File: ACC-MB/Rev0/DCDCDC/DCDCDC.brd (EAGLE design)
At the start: 99 x 78 mm, 20 parts, among them X5 5566-8

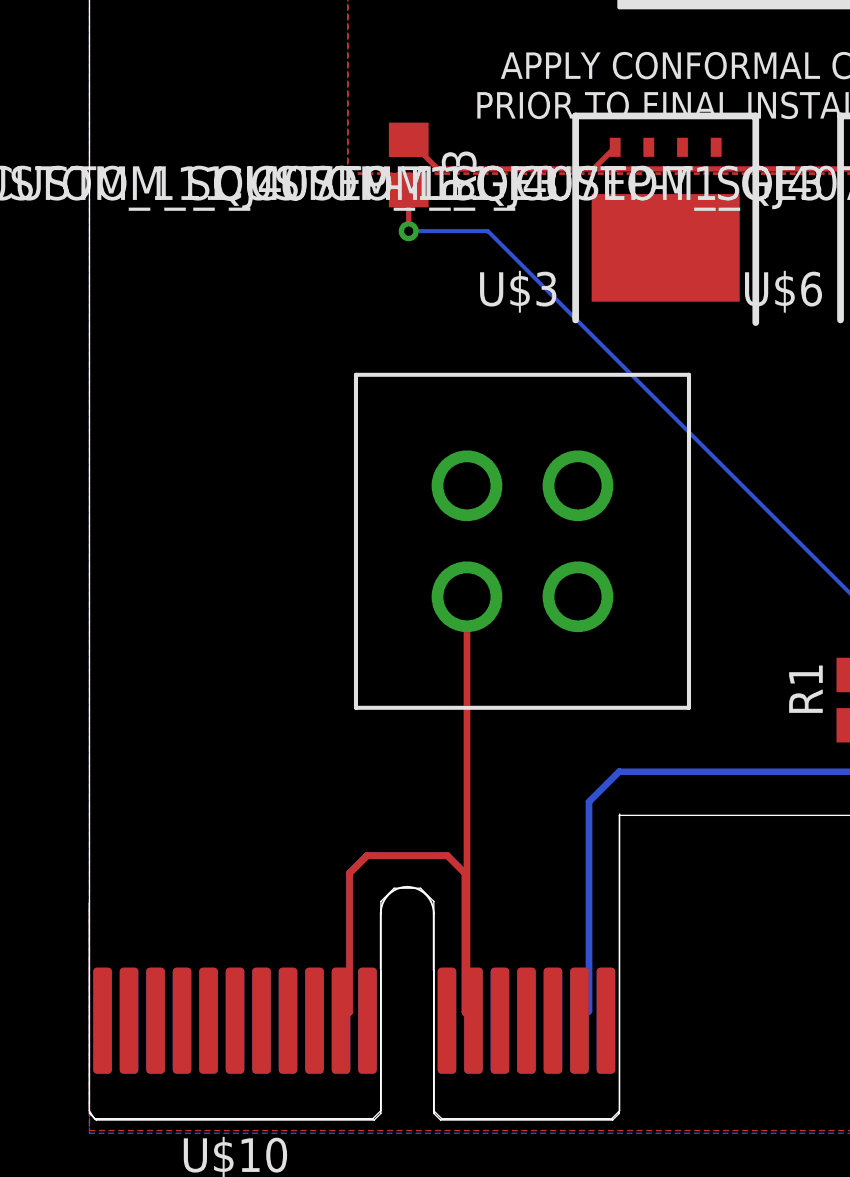
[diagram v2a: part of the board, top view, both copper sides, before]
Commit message: update
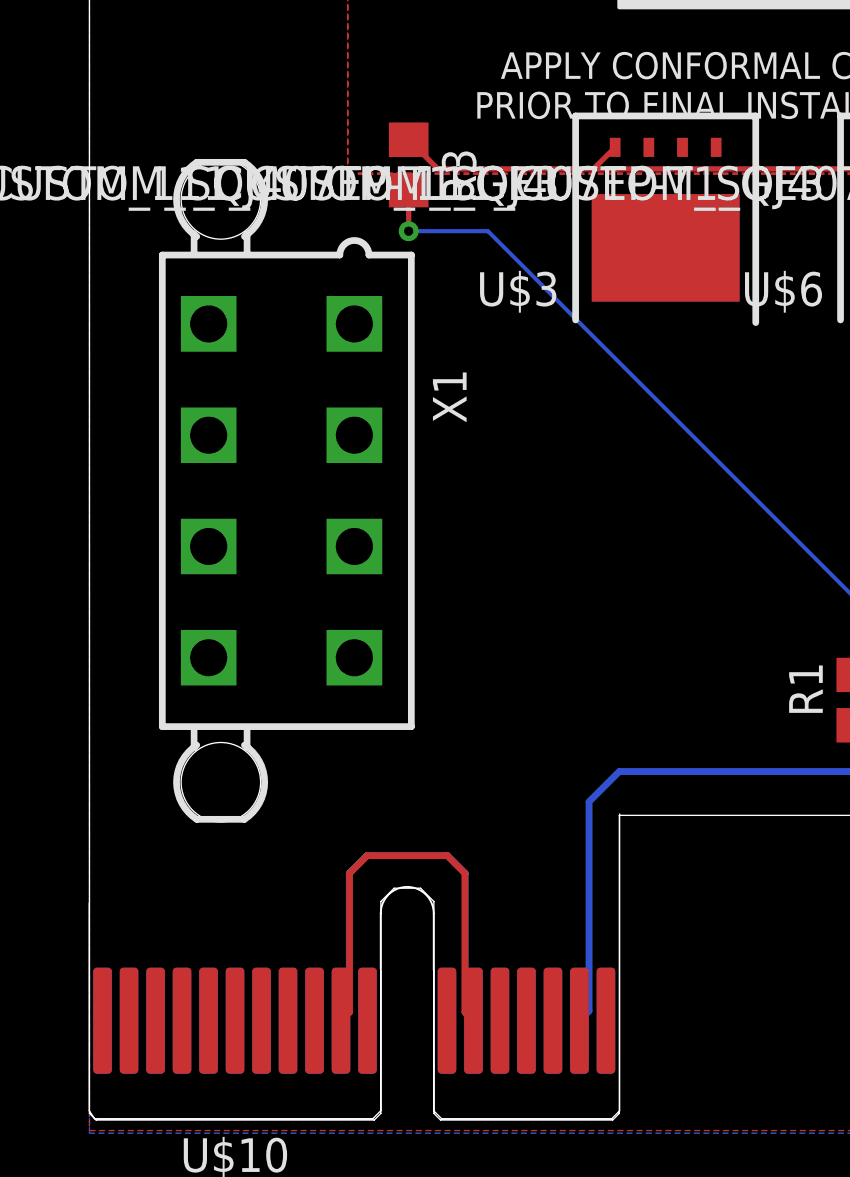
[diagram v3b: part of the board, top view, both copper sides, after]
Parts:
- removed U$1: IPBT-102-H1-T-D, ACC-MB-R0:IPBT-102-H1-T-D
- added X1: 5566-8, con-molex:5566-8
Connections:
- new net N$5: X1.1, X1.2, X1.5
- new net N$6: X1.4, X1.7, X1.8
- net +12V: no longer U$1.P$1, U$1.P$2
- net GND: no longer U$1.P$3, U$1.P$4
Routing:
- net +12V: track 36.6 -> 20.8 mm
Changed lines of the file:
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@@
 <element name="U$3" library="PDM_2019_RevB" package="_CUSTOM_111_CUSTOM_TRANS_SIRA90DP-T1-GE3" value="_CUSTOM_111_CUSTOM_SQJ407EP-T1_GE3" x="22" y="22.5" rot="R180"/>
 <element name="U$10" library="ACC-MB-R0" library_urn="urn:adsk.eagle:library:13324935" package="PCI-E_SLOT_36" value="PCIE-36-EDGE" x="0.5" y="-11.5"/>
-<element name="U$1" library="ACC-MB-R0" library_urn="urn:adsk.eagle:library:13324935" package="IPBT-102-H1-T-D" package3d_urn="urn:adsk.eagle:package:13324986/2" value="IPBT-102-H1-T-D" x="14.5" y="8.25"/>
 <element name="U$2" library="ACC-MB-R0" library_urn="urn:adsk.eagle:library:13324935" package="PCI-E_SLOT_36" value="PCIE-36-EDGE" x="79.5" y="-11.5"/>
 <element name="X5" library="con-molex" library_urn="urn:adsk.eagle:library:165" package="5566-8" value="5566-8" x="84" y="58.75">
@@
 <attribute name="OC_FARNELL" value="unknown" x="84" y="58.75" size="1.778" layer="27" display="off"/>
 <attribute name="OC_NEWARK" value="unknown" x="84" y="58.75" size="1.778" layer="27" display="off"/>
+</element>
+<element name="X1" library="con-molex" library_urn="urn:adsk.eagle:library:165" package="5566-8" value="5566-8" x="7.5" y="12.25" rot="R90">
+<attribute name="MF" value="MOLEX" x="7.5" y="12.25" size="1.778" layer="27" rot="R90" display="off"/>
+<attribute name="MPN" value="" x="7.5" y="12.25" size="1.778" layer="27" rot="R90" display="off"/>
+<attribute name="OC_FARNELL" value="unknown" x="7.5" y="12.25" size="1.778" layer="27" rot="R90" display="off"/>
+<attribute name="OC_NEWARK" value="unknown" x="7.5" y="12.25" size="1.778" layer="27" rot="R90" display="off"/>
 </element>
 </elements>
@@
 <wire x1="34.35" y1="2.35" x2="30.25" y2="2.35" width="0.2" layer="1"/>
 <wire x1="44.2" y1="1.65" x2="46" y2="1.65" width="0.2" layer="1"/>
-<contactref element="U$1" pad="P$4"/>
-<contactref element="U$1" pad="P$3"/>
 <contactref element="U$10" pad="A2"/>
 <contactref element="U$10" pad="A3"/>
@@
 <wire x1="10.0565" y1="-7.4385" x2="10.0565" y2="-2.18105625" width="0.254" layer="16"/>
 <wire x1="14.4335" y1="-2.18105625" x2="14.4335" y2="-7.4385" width="0.254" layer="16"/>
+<wire x1="21.16" y1="45.25" x2="21.16" y2="56.25" width="0" layer="19" extent="1-1"/>
+<wire x1="6.19" y1="55" x2="21.16" y2="56.25" width="0" layer="19" extent="1-1"/>
+<wire x1="29.2" y1="3.4" x2="21.16" y2="45.25" width="0" layer="19" extent="1-1"/>
+<wire x1="17.745" y1="-7.75" x2="18.745" y2="-7.75" width="0" layer="19" extent="16-16"/>
+<wire x1="16.745" y1="-7.75" x2="17.745" y2="-7.75" width="0" layer="19" extent="16-16"/>
+<wire x1="15.745" y1="-7.75" x2="16.745" y2="-7.75" width="0" layer="19" extent="16-16"/>
+<wire x1="14.745" y1="-7.75" x2="15.745" y2="-7.75" width="0" layer="19" extent="16-16"/>
+<wire x1="8.745" y1="-7.75" x2="9.745" y2="-7.75" width="0" layer="19" extent="16-16"/>
+<wire x1="7.745" y1="-7.75" x2="8.745" y2="-7.75" width="0" layer="19" extent="16-16"/>
+<wire x1="6.745" y1="-7.75" x2="7.745" y2="-7.75" width="0" layer="19" extent="16-16"/>
+<wire x1="5.745" y1="-7.75" x2="6.745" y2="-7.75" width="0" layer="19" extent="16-16"/>
+<wire x1="4.745" y1="-7.75" x2="5.745" y2="-7.75" width="0" layer="19" extent="16-16"/>
+<wire x1="3.745" y1="-7.75" x2="4.745" y2="-7.75" width="0" layer="19" extent="16-16"/>
+<wire x1="2.745" y1="-7.75" x2="3.745" y2="-7.75" width="0" layer="19" extent="16-16"/>
+<wire x1="1.745" y1="-7.75" x2="2.745" y2="-7.75" width="0" layer="19" extent="16-16"/>
 </signal>
 <signal name="V+" class="1">
@@
 <contactref element="U$6" pad="5"/>
 <contactref element="U$3" pad="5"/>
-<contactref element="U$1" pad="P$2"/>
-<contactref element="U$1" pad="P$1"/>
 <contactref element="U$10" pad="B2"/>
 <contactref element="U$10" pad="B3"/>
@@
 <contactref element="U$10" pad="B16"/>
 <contactref element="U$10" pad="B17"/>
-<wire x1="14.5" y1="8.25" x2="14.5" y2="-7.505" width="0.254" layer="1"/>
 <wire x1="14.5" y1="-7.505" x2="14.745" y2="-7.75" width="0.254" layer="1"/>
 <wire x1="10.067" y1="-2.19155625" x2="10.73655625" y2="-1.522" width="0.254" layer="1"/>
@@
 <wire x1="10.067" y1="-7.428" x2="10.067" y2="-2.19155625" width="0.254" layer="1"/>
 <wire x1="14.423" y1="-2.19155625" x2="14.423" y2="-7.428" width="0.254" layer="1"/>
+<wire x1="32" y1="21.42" x2="42" y2="21.42" width="0" layer="19" extent="1-1"/>
+<wire x1="22" y1="21.42" x2="32" y2="21.42" width="0" layer="19" extent="1-1"/>
+<wire x1="39.8" y1="4.45" x2="42" y2="21.42" width="0" layer="19" extent="1-1"/>
+<wire x1="18.745" y1="-7.75" x2="38.15" y2="3.15" width="0" layer="19" extent="1-1"/>
+<wire x1="17.745" y1="-7.75" x2="18.745" y2="-7.75" width="0" layer="19" extent="1-1"/>
+<wire x1="16.745" y1="-7.75" x2="17.745" y2="-7.75" width="0" layer="19" extent="1-1"/>
+<wire x1="15.745" y1="-7.75" x2="16.745" y2="-7.75" width="0" layer="19" extent="1-1"/>
+<wire x1="14.745" y1="-7.75" x2="15.745" y2="-7.75" width="0" layer="19" extent="1-1"/>
+<wire x1="8.745" y1="-7.75" x2="9.745" y2="-7.75" width="0" layer="19" extent="1-1"/>
+<wire x1="7.745" y1="-7.75" x2="8.745" y2="-7.75" width="0" layer="19" extent="1-1"/>
+<wire x1="6.745" y1="-7.75" x2="7.745" y2="-7.75" width="0" layer="19" extent="1-1"/>
+<wire x1="5.745" y1="-7.75" x2="6.745" y2="-7.75" width="0" layer="19" extent="1-1"/>
+<wire x1="4.745" y1="-7.75" x2="5.745" y2="-7.75" width="0" layer="19" extent="1-1"/>
+<wire x1="3.745" y1="-7.75" x2="4.745" y2="-7.75" width="0" layer="19" extent="1-1"/>
+<wire x1="2.745" y1="-7.75" x2="3.745" y2="-7.75" width="0" layer="19" extent="1-1"/>
+<wire x1="1.745" y1="-7.75" x2="2.745" y2="-7.75" width="0" layer="19" extent="1-1"/>
 </signal>
 <signal name="N$2">
@@
 <wire x1="19.28" y1="24.4" x2="19.25" y2="24.4" width="0.2032" layer="1"/>
 </signal>
+<signal name="N$5" class="1">
+<contactref element="X1" pad="1"/>
+<contactref element="X1" pad="5"/>
+<contactref element="X1" pad="2"/>
+<wire x1="10.25" y1="18.55" x2="10.25" y2="14.35" width="0" layer="19" extent="1-1"/>
+<wire x1="4.75" y1="18.55" x2="10.25" y2="18.55" width="0" layer="19" extent="1-1"/>
+</signal>
+<signal name="N$6" class="1">
+<contactref element="X1" pad="8"/>
+<contactref element="X1" pad="4"/>
+<contactref element="X1" pad="7"/>
+<wire x1="4.75" y1="5.95" x2="10.25" y2="5.95" width="0" layer="19" extent="1-1"/>
+<wire x1="4.75" y1="10.15" x2="4.75" y2="5.95" width="0" layer="19" extent="1-1"/>
+</signal>
 </signals>
